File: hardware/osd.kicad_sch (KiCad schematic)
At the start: 12 parts, among them U14 SN74LVC1G3157, U15 TLV7031

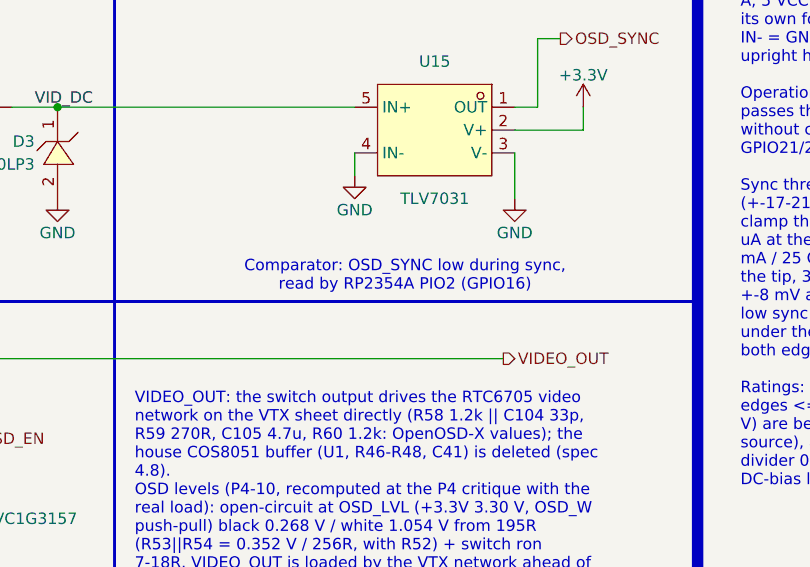
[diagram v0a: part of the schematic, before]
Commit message: WIP final schematic (D111/D113): further sheet and doc updates, PDF re-export; mid-run snapshot, not yet verified
Co-Authored-By: Claude Opus 5.5 <noreply@anthropic.com>
Claude-Session: https://claude.ai/code/session_01RFaS5jnC9tnPam9GBgmGnG
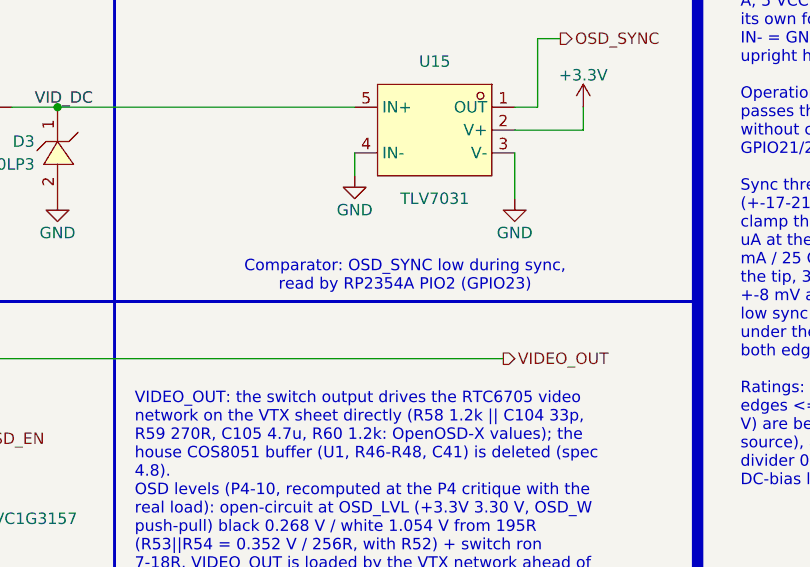
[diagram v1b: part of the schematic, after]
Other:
- note added: "Comparator: OSD_SYNC low during sync, read by RP2354A PIO2 (GPIO23)"
- note removed: "Comparator: OSD_SYNC low during sync, read by RP2354A PIO2 (GPIO16)"
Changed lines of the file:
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@@
 		)
 	)
-	(text "Comparator: OSD_SYNC low during sync,\nread by RP2354A PIO2 (GPIO16)"
+	(text "Comparator: OSD_SYNC low during sync,\nread by RP2354A PIO2 (GPIO23)"
 		(exclude_from_sim no)
 		(at 164.338 74.676 0)
